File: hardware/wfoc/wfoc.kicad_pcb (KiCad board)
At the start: 2 copper layers, 50 x 50 mm, 70 parts, among them Q1 NMOS, Q2 NMOS, Q3 NMOS, Q4 NMOS, Q5 NMOS, Q6 NMOS, U3 TSSOP20, U4 6209

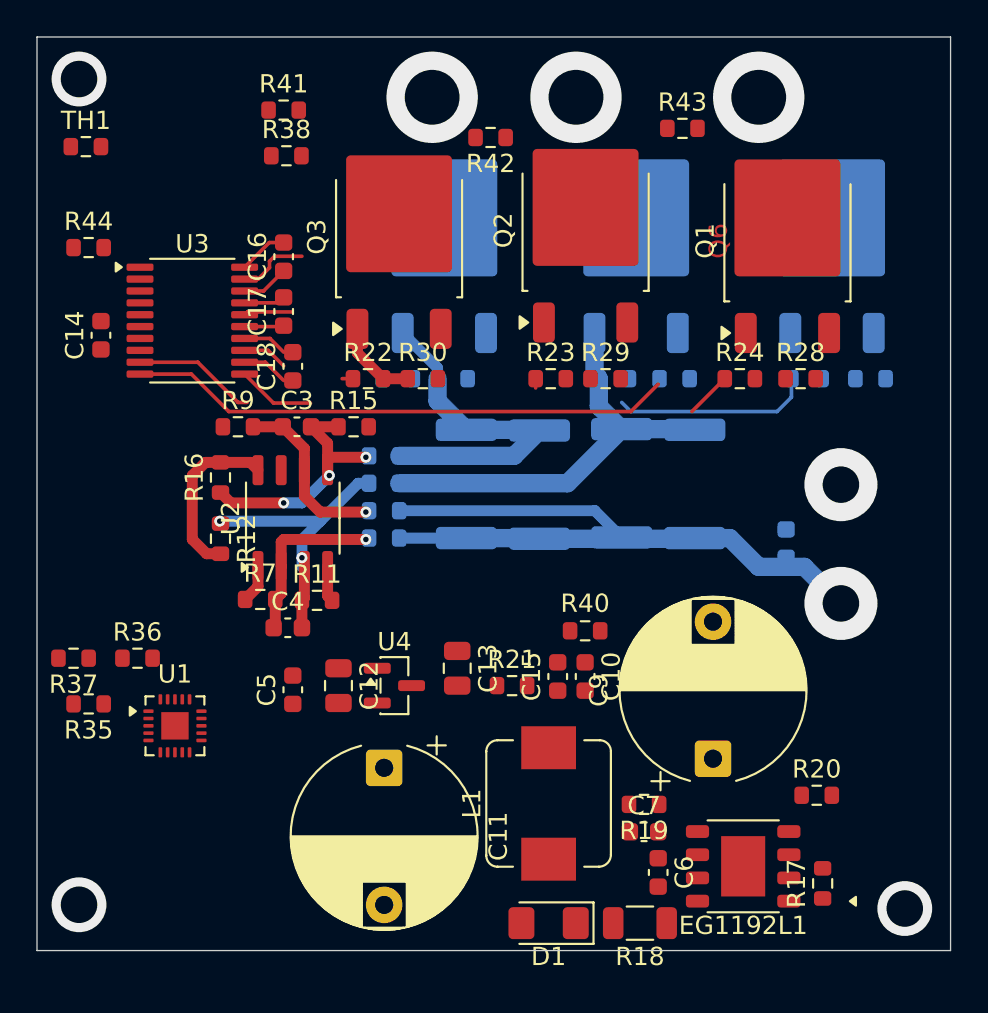
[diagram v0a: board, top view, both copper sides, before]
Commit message: save last vesion
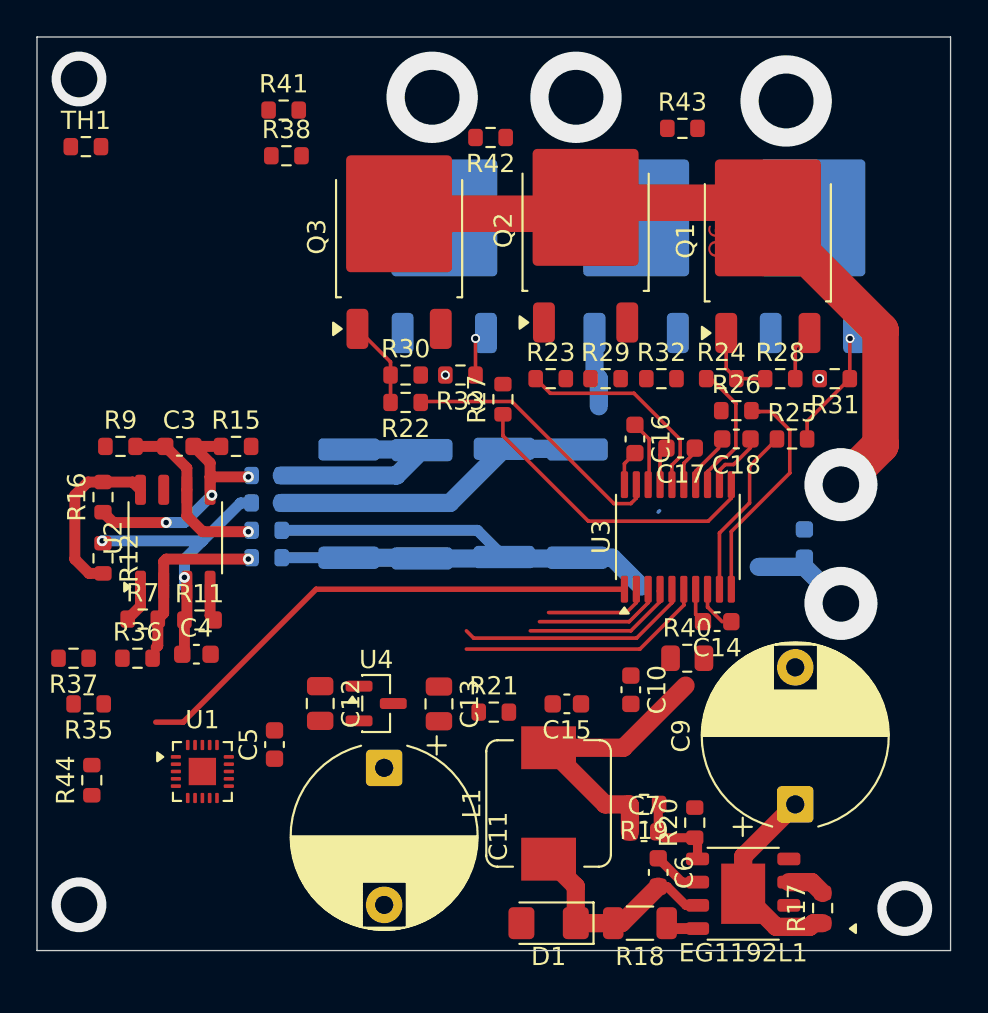
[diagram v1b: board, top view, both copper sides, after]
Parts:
- R25, R26, R27, R31, R32, R33: moved to F.Cu
- R40: value 10K -> 47K; footprint Resistor_SMD:R_0603_1608Metric -> Resistor_SMD:R_0805_2012Metric
- moved C14 37.2 mm to (154.7, 95.0), turned to 180 degrees
- moved R44 29.2 mm to (120.5, 103.7), turned to 90 degrees
- moved U3 29.1 mm to (152.6, 90.4), turned to 90 degrees
- moved C18 24.6 mm to (155.8, 85.0), turned to 180 degrees
- moved C17 23.0 mm to (152.7, 85.5), turned to 180 degrees
- moved C16 21.7 mm to (150.2, 85.0), turned to -90 degrees
- moved R20 6.84 mm to (153.5, 106.0), turned to 90 degrees
- moved R10 6.52 mm to (130.1, 90.0)
- moved R12 6.52 mm to (121.1, 91.5)
- moved R16 6.52 mm to (121.1, 88.2)
- moved R2 6.52 mm to (138.6, 88.6)
- moved R3 6.52 mm to (130.1, 87.0)
- moved R4 6.52 mm to (143.1, 88.5)
- moved R5 6.52 mm to (130.1, 88.5)
- moved R8 6.52 mm to (130.1, 91.5)
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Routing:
- net +BATT: track 0.00 -> 55.3 mm
- net PWM_AH: track 0.00 -> 28.7 mm
- net +12V: track 0.00 -> 18.3 mm
- net Net-(U3-LO2): track 29.8 -> 13.3 mm
- net PWM_CL: track 0.00 -> 13.8 mm
- net Net-(D1-K): track 0.00 -> 13.2 mm
- net PWM_BL: track 0.00 -> 13.0 mm
- net Net-(U3-LO1): track 4.26 -> 16.9 mm
- net Net-(U3-HO1): track 4.45 -> 15.0 mm
- net Net-(U3-HO2): track 3.18 -> 11.9 mm
- net PWM_AL: track 0.00 -> 8.58 mm
- net Net-(U3-LO3): track 17.6 -> 9.53 mm
- net PWM_CH: track 0.00 -> 7.12 mm
- net Ia_P: track 19.0 -> 12.3 mm, vias 0 -> 1
- net LO3: track 0.00 -> 6.47 mm, vias 0 -> 1
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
